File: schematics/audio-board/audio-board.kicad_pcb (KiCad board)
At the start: 2 copper layers, 59.5 x 19 mm, 17 parts, among them J3 Conn_01x04, J4 Conn_Coaxial_Power, SW1 5V_BYPASS, U1 Teensy4.0, U2 spdif_recv, U3 LM1117-5, U5 S-2151, U6 VN7140

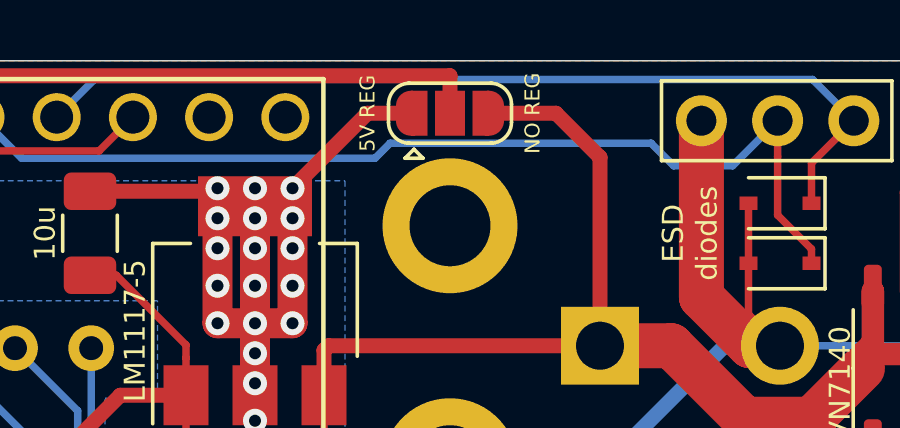
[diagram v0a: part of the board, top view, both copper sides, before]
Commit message: ok
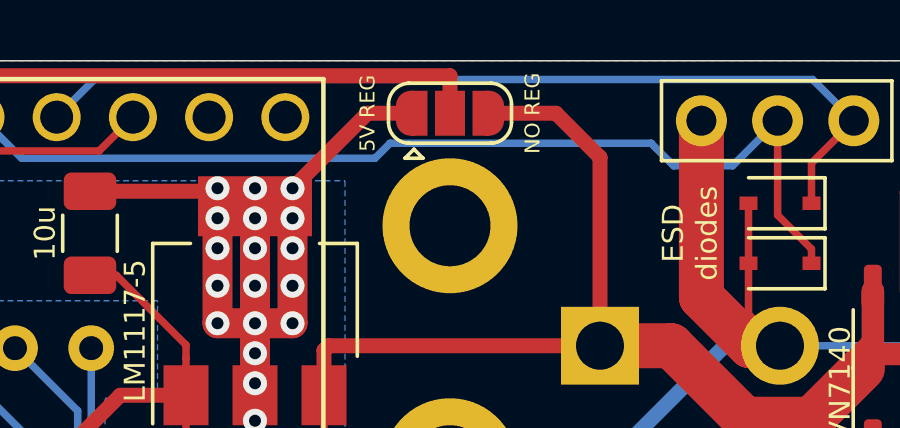
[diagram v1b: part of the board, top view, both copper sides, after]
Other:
- net class 50V removed
- net class Default removed
- net class HV removed
